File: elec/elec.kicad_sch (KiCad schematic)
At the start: 34 parts, among them J1 DB301V-3.5-2P-GN-S, J2 BM04B-SRSS-TB, SW1 YTSA010, U1 MCP23017_SP

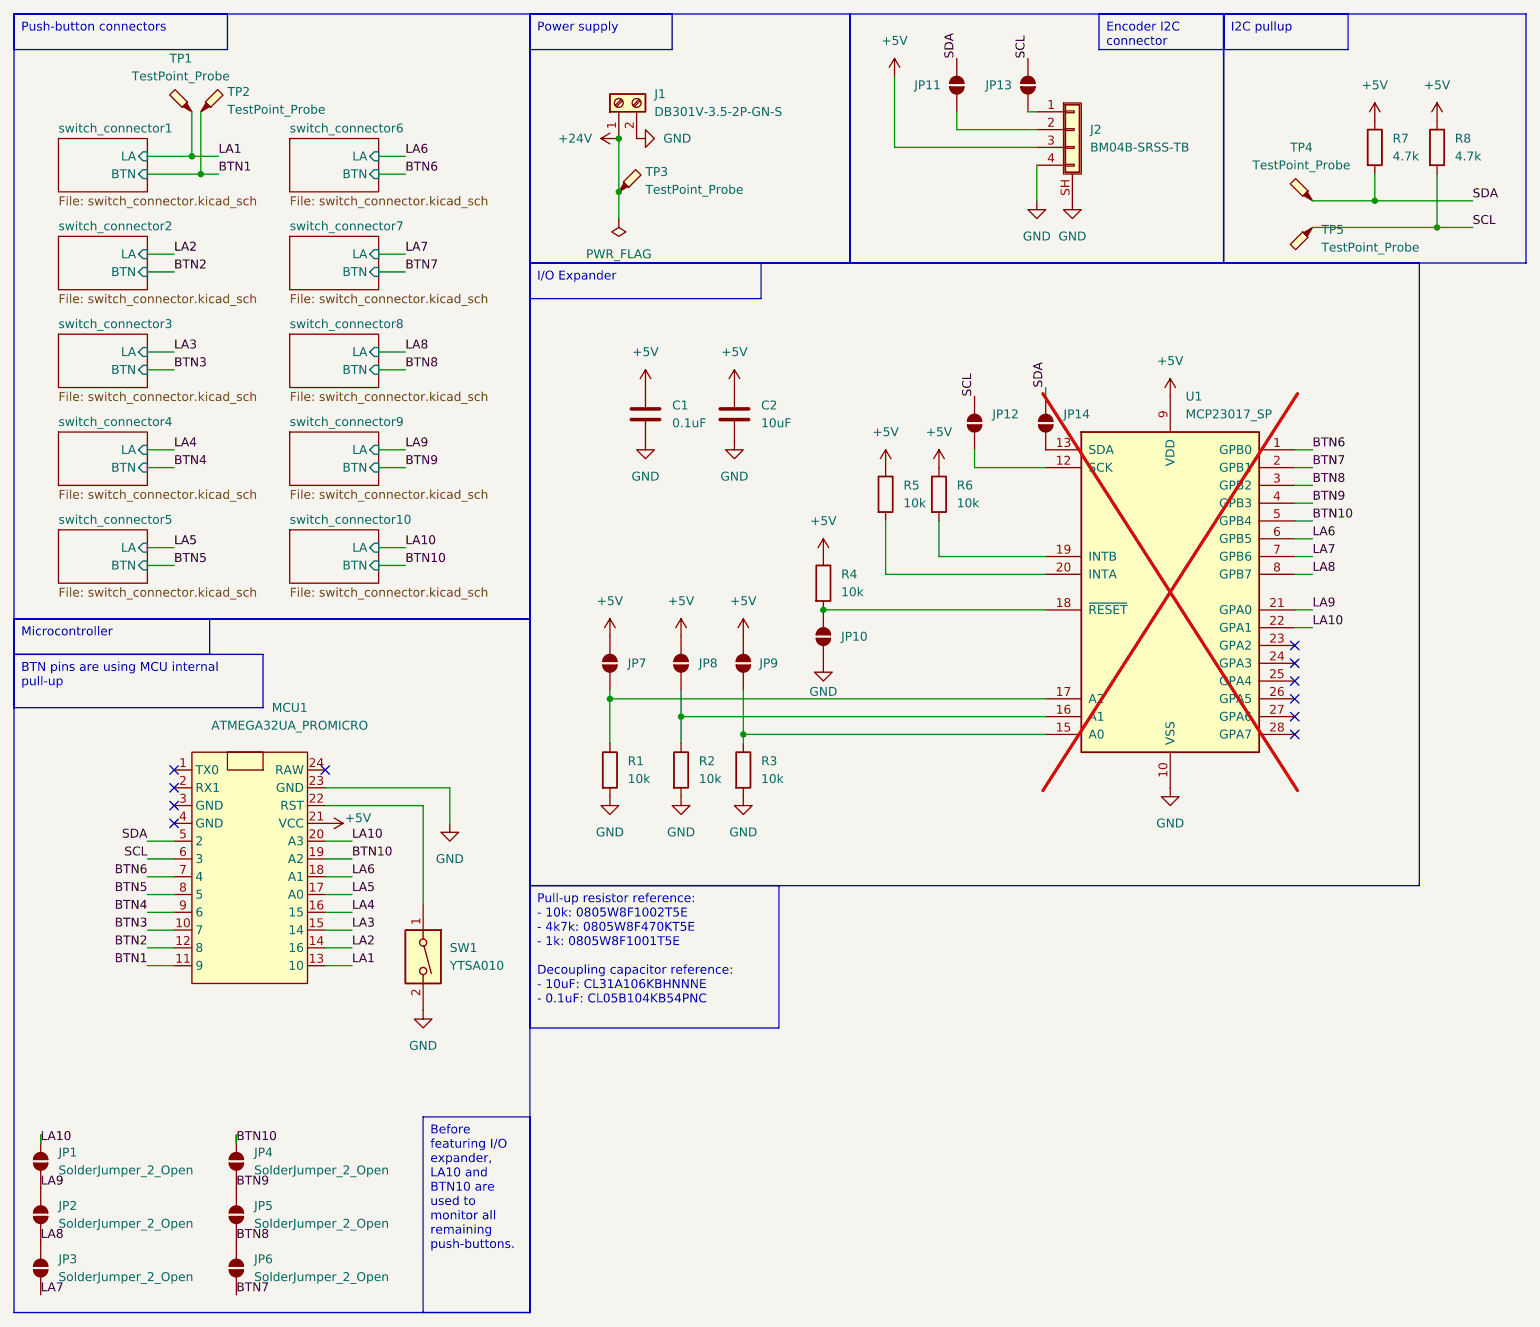
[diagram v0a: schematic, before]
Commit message: v1 3D print PCB
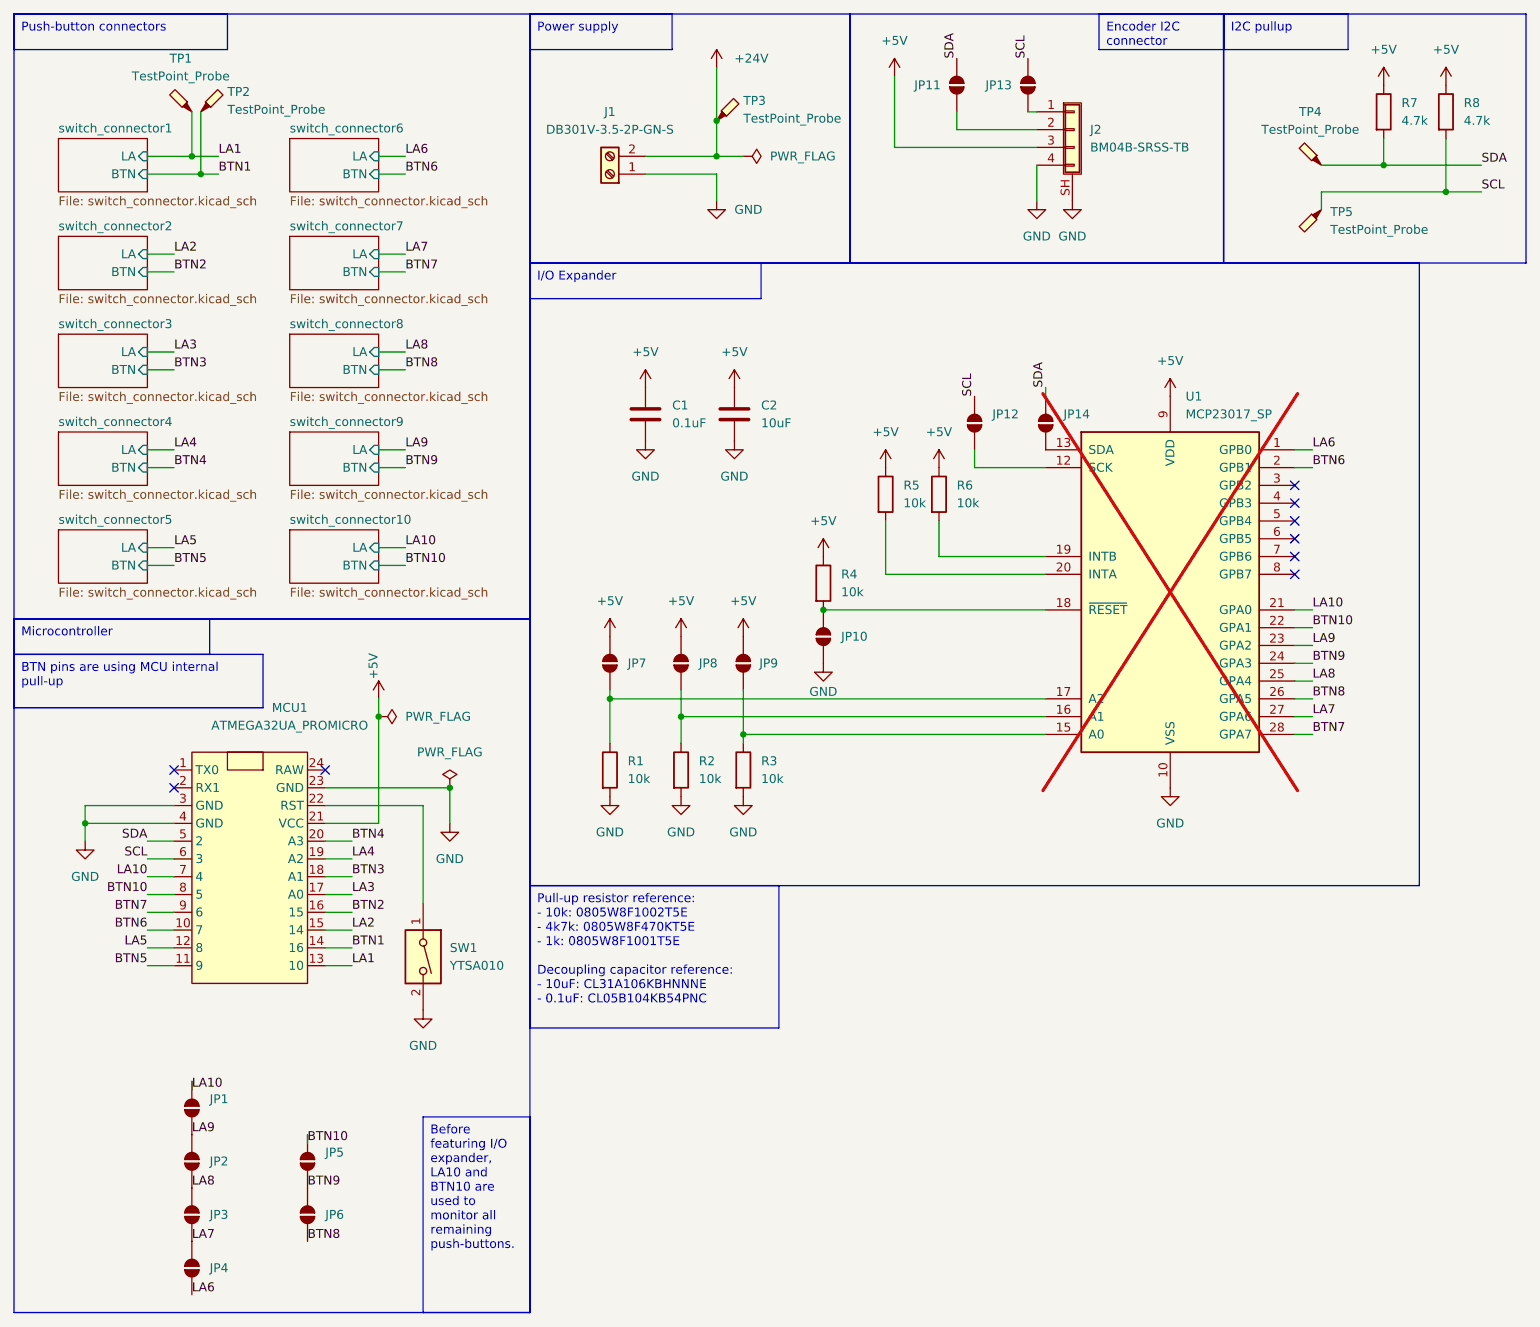
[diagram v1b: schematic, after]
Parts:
- renumbered JP6 to JP4, JP4 to JP5, JP5 to JP6
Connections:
- net +24V: now also J1.2 (Pin_2); no longer J1.1 (Pin_1)
- net BTN1: now also MCU1.14 (16); no longer MCU1.11 (9)
- net BTN10: now also MCU1.8 (5), U1.22 (GPA1); no longer MCU1.19 (A2), U1.5 (GPB4)
- net BTN2: now also MCU1.16 (15); no longer MCU1.12 (8)
- net BTN3: now also MCU1.18 (A1); no longer MCU1.10 (7)
- net BTN4: now also MCU1.20 (A3); no longer MCU1.9 (6)
- net BTN5: now also MCU1.11 (9); no longer MCU1.8 (5)
- net BTN6: now also MCU1.10 (7), U1.2 (GPB1); no longer MCU1.7 (4), U1.1 (GPB0)
- net BTN7: now also MCU1.9 (6), U1.28 (GPA7); no longer JP4.1 (A), U1.2 (GPB1)
- net BTN8: now also U1.26 (GPA5); no longer JP4.2 (B), U1.3 (GPB2)
- net BTN9: now also U1.24 (GPA3); no longer U1.4 (GPB3)
- net GND: now also J1.1 (Pin_1), MCU1.3 (GND), MCU1.4 (GND); no longer J1.2 (Pin_2)
- net LA10: now also MCU1.7 (4), U1.21 (GPA0); no longer MCU1.20 (A3), U1.22 (GPA1)
- net LA2: now also MCU1.15 (14); no longer MCU1.14 (16)
- net LA3: now also MCU1.17 (A0); no longer MCU1.15 (14)
- net LA4: now also MCU1.19 (A2); no longer MCU1.16 (15)
- net LA5: now also MCU1.12 (8); no longer MCU1.17 (A0)
- net LA6: now also JP4.1 (A), U1.1 (GPB0); no longer MCU1.18 (A1), U1.6 (GPB5)
- net LA7: now also JP4.2 (B), U1.27 (GPA6); no longer U1.7 (GPB6)
- net LA8: now also U1.25 (GPA4); no longer U1.8 (GPB7)
- net LA9: now also U1.23 (GPA2); no longer U1.21 (GPA0)
- no-connect marks 11 -> 9
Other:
- moved on the sheet: J1, JP1, JP2, JP3, JP4, JP5, JP6, R7, R8, TP3, TP4, TP5
